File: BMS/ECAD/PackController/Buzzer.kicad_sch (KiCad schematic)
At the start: 5 parts, among them Q801 2N7002

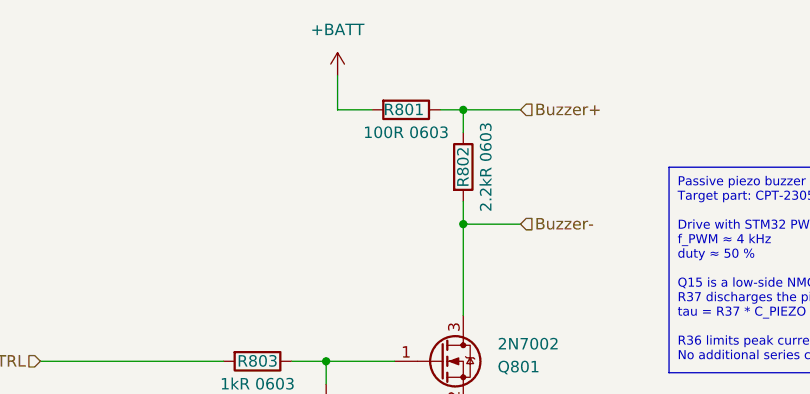
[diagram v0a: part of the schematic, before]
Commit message: many fixes
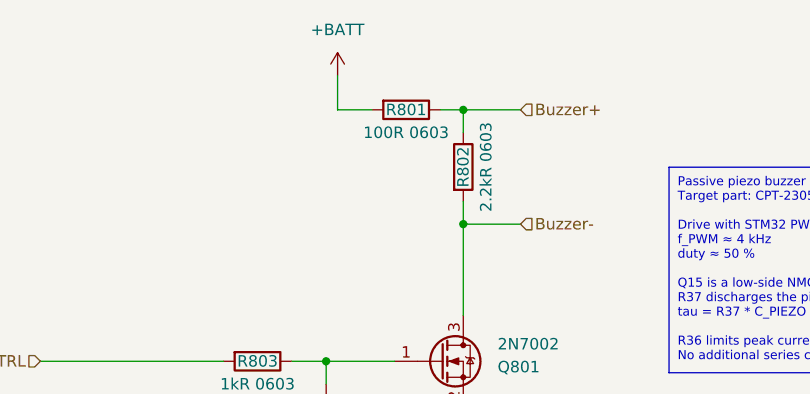
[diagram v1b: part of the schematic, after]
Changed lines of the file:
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@@
 		(dnp no)
 		(property "Reference" "R801"
-			(at 138.176 72.39 90)
+			(at 138.43 72.39 90)
 			(show_name no)
 			(do_not_autoplace no)
